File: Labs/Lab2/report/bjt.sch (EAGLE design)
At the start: 32 parts, among them Q1 2N3906, Q2 2N3906

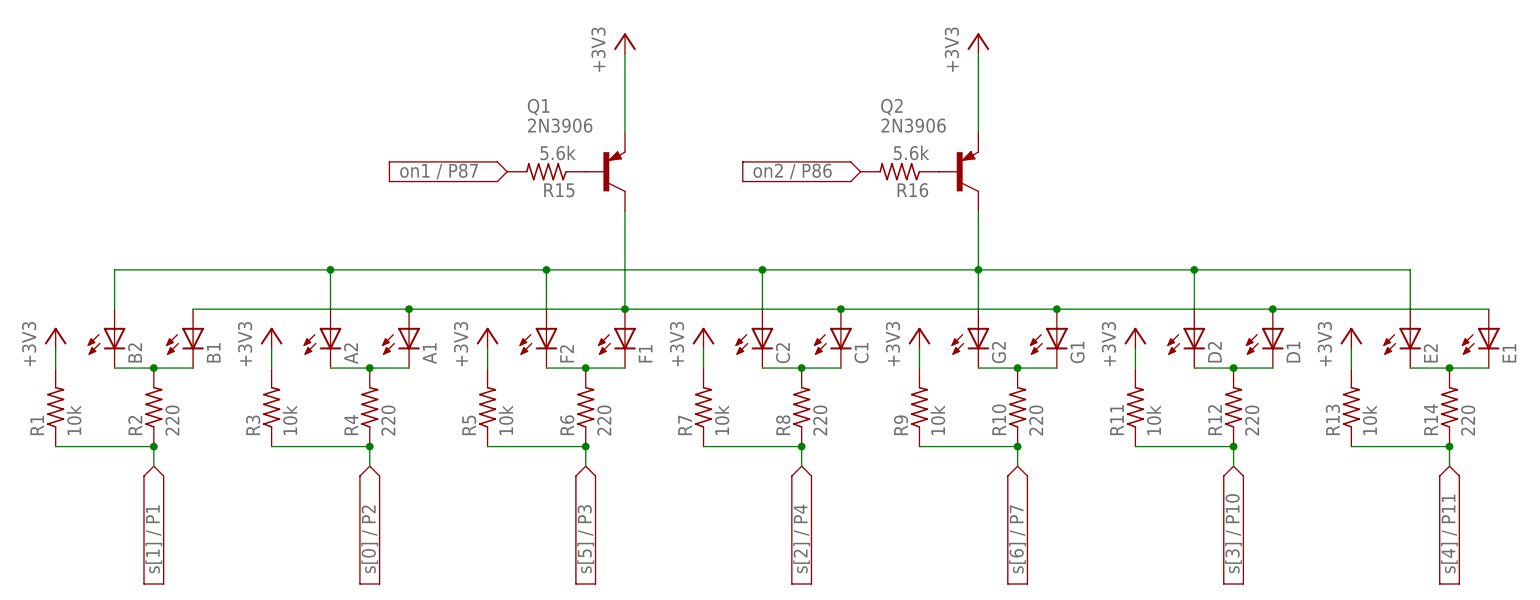
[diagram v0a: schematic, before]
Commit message: Finished lab report 2
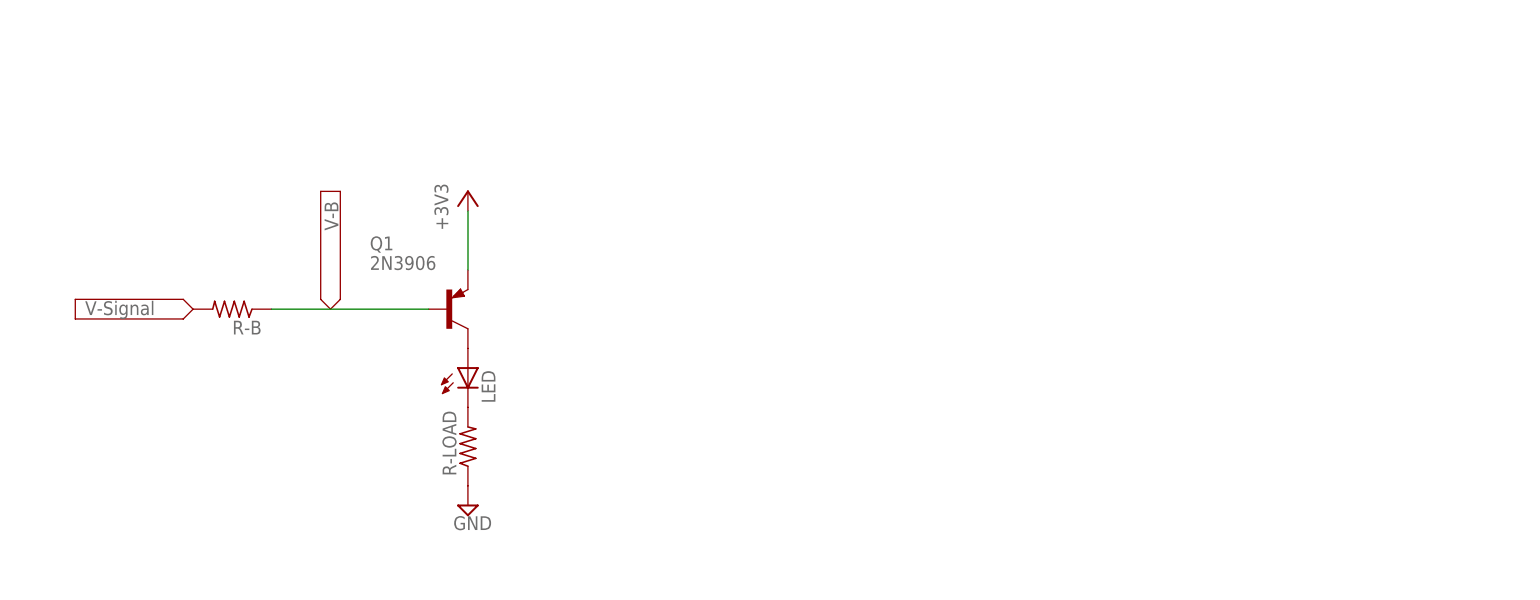
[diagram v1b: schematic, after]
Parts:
- removed A1, A2, B1, B2, C1, C2, D1, D2, E1, E2, F1, F2, G1, G2: (no value), adafruit:LED5MM
- removed Q2: 2N3906, transistor-pnp:2N3906
- removed R1, R11, R13, R3, R5, R7, R9: 10k, resistor:R-US_0411/12
- removed R10, R12, R14, R2, R4, R6, R8: 220, resistor:R-US_0411/12
- removed R15, R16: 5.6k, resistor:R-US_0411/12
- added LED: (no value), adafruit:LED5MM
- added R-B, R-LOAD: (no value), resistor:R-US_0411/12
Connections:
- removed net A1: A1.C, A2.C, R4.2
- removed net N$10: C1.C, C2.C, R8.2
- removed net N$11: R7.1, R8.1
- removed net N$13: G1.C, G2.C, R10.2
- removed net N$14: R10.1, R9.1
- removed net N$17: D1.C, D2.C, R12.2
- removed net N$18: R11.1, R12.1
- removed net N$2: B1.C, B2.C, R2.2
- removed net N$20: E1.C, E2.C, R14.2
- removed net N$21: R13.1, R14.1
- removed net N$3: R1.1, R2.1
- removed net N$5: R3.1, R4.1
- removed net N$6: A1.A, B1.A, C1.A, D1.A, E1.A, F1.A, G1.A, Q1.C
- removed net N$7: F1.C, F2.C, R6.2
- removed net N$9: Q2.B, R16.1
- new net GND: R-LOAD.1
- net +3V3: no longer Q2.E, R1.2, R11.2, R13.2, R3.2, R5.2, R7.2, R9.2
- net N$1: now also LED.A, Q1.C; no longer A2.A, B2.A, C2.A, D2.A, E2.A, F2.A, G2.A, Q2.C
- net N$16: now also R-B.1; no longer R15.1
- net N$8: now also LED.C, R-LOAD.2; no longer R5.1, R6.1
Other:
- moved on the sheet: Q1
